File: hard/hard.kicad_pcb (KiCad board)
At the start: 2 copper layers, 315.6 x 117.5 mm, 177 parts, among them J1 USB_C_Receptacle_USB2.0, J2 RJ45_Shielded, J3 RJ45_Shielded, SW1 BOOT0, SW2 BOOT1, SW3 BOOT0, SW4 BOOT1, U1 STM32F401RETx, U2 USBLC6-2SC6, U3 AMS1117-3.3, U4 STM32F401RETx, Y1 XTAL_8M, Y3 XTAL_8M

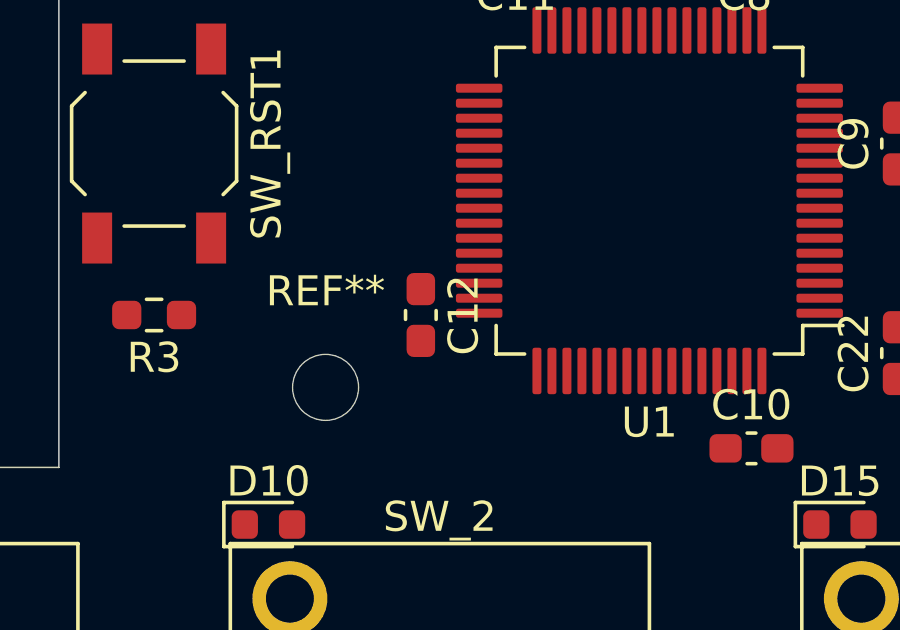
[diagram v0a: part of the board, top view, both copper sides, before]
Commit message: misc circuits
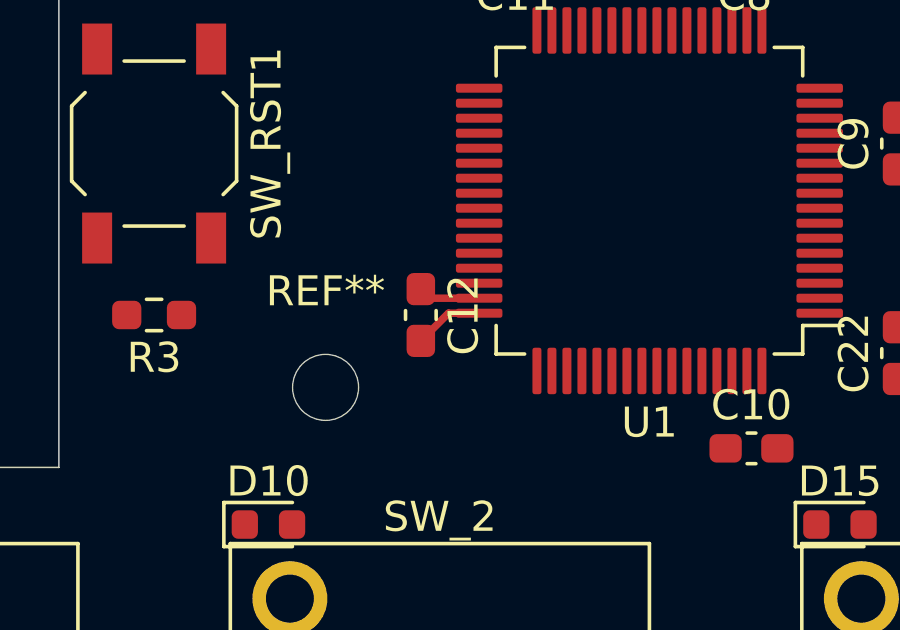
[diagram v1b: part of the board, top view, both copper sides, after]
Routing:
- net +3V3: track 0.00 -> 2.33 mm
- net GND: track 0.00 -> 2.07 mm

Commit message: gen2
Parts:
- removed C15, C17, C19, C20, C21, C22, C23: 0.1uF, Capacitor_SMD:C_0603_1608Metric_Pad1.08x0.95mm_HandSolder
- removed C16: 10uF, Capacitor_SMD:C_0603_1608Metric_Pad1.08x0.95mm_HandSolder
- removed C18: 4.7uF, Capacitor_SMD:C_0603_1608Metric_Pad1.08x0.95mm_HandSolder
- removed C24, C25: 12pF, Capacitor_SMD:C_0603_1608Metric_Pad1.08x0.95mm_HandSolder
- removed D10, D11, D12, D13, D14, D15, D16, D17, D18, D19, D20, D21, D22, D23, D24, D25, D26, D27, D29, D30, D31, D32, D33, D34, D35, D36, D37, D38, D39, D4, D40, D41, D42, D43, D44, D45, D46, D47, D48, D49, D5, D50, D51, D52, D53, D54, D55, D56, D57, D58, D59, D6, D60, D61, D62, D7, D8, D9: D, Diode_SMD:D_0603_1608Metric
- removed J3: RJ45_Shielded, Connector_RJ:RJ45_Ninigi_GE
- removed REF** (x8): MountingHole_2.2mm_M2, MountingHole:MountingHole_2.2mm_M2
- removed SW_0: SW_0, hard:Kailh_Choc_V2_1.00u_PCB
- removed SW_1: SW_1, hard:Kailh_Choc_V2_1.00u_PCB
- removed SW_10: SW_6, hard:Kailh_Choc_V2_1.00u_PCB
- removed SW_2: SW_2, hard:Kailh_Choc_V2_1.00u_PCB
- removed SW_3: SW_3, hard:Kailh_Choc_V2_1.00u_PCB
- removed SW_4: SW_4, hard:Kailh_Choc_V2_1.00u_PCB
- removed SW_5: SW_5, hard:Kailh_Choc_V2_1.00u_PCB
- removed SW_7: SW_7, hard:Kailh_Choc_V2_1.00u_PCB
- removed SW_8: SW_8, hard:Kailh_Choc_V2_1.00u_PCB
- removed SW_9: SW_9, hard:Kailh_Choc_V2_1.00u_PCB
- removed SW_A1: SW_A, hard:Kailh_Choc_V2_1.00u_PCB
- removed SW_B1: SW_B, hard:Kailh_Choc_V2_1.00u_PCB
- removed SW_BQ1: SW_BQ, hard:Kailh_Choc_V2_1.00u_PCB
- removed SW_BS1: SW_BS, hard:Kailh_Choc_V2_1.50u_PCB
- removed SW_C1: SW_C, hard:Kailh_Choc_V2_1.00u_PCB
- removed SW_CMM1: SW_CMM, hard:Kailh_Choc_V2_1.00u_PCB
- removed SW_CTRL1: SW_CTRL, hard:Kailh_Choc_V2_1.75u_PCB
- removed SW_D1: SW_D, hard:Kailh_Choc_V2_1.00u_PCB
- removed SW_DEL1: SW_DEL, hard:Kailh_Choc_V2_2.00u_PCB
- removed SW_E1: SW_E, hard:Kailh_Choc_V2_1.00u_PCB
- removed SW_ESC1: SW_ESC, hard:Kailh_Choc_V2_1.00u_PCB
- removed SW_F1: SW_F, hard:Kailh_Choc_V2_1.00u_PCB
- removed SW_FN1: SW_FN, hard:Kailh_Choc_V2_1.00u_PCB
- removed SW_G1: SW_G, hard:Kailh_Choc_V2_1.00u_PCB
- removed SW_H1: SW_H, hard:Kailh_Choc_V2_1.00u_PCB
- removed SW_HYPH1: SW_HYPH, hard:Kailh_Choc_V2_1.00u_PCB
- removed SW_I1: SW_I, hard:Kailh_Choc_V2_1.00u_PCB
- removed SW_J1: SW_J, hard:Kailh_Choc_V2_1.00u_PCB
- removed SW_K1: SW_K, hard:Kailh_Choc_V2_1.00u_PCB
- removed SW_L1: SW_L, hard:Kailh_Choc_V2_1.00u_PCB
- removed SW_LALT1: SW_LALT, hard:Kailh_Choc_V2_1.25u_PCB
- removed SW_LB1: SW_LB, hard:Kailh_Choc_V2_1.00u_PCB
- removed SW_LCMD1: SW_LCMD, hard:Kailh_Choc_V2_1.25u_PCB
- removed SW_LSFT1: SW_LSFT, hard:Kailh_Choc_V2_2.25u_PCB
- removed SW_LSPC1: SW_LSPC, hard:Kailh_Choc_V2_2.00u_PCB
- removed SW_M1: SW_M, hard:Kailh_Choc_V2_1.00u_PCB
- removed SW_N1: SW_N, hard:Kailh_Choc_V2_1.00u_PCB
- removed SW_O1: SW_O, hard:Kailh_Choc_V2_1.00u_PCB
- removed SW_P1: SW_P, hard:Kailh_Choc_V2_1.00u_PCB
- removed SW_PLUS1: SW_PLUS, hard:Kailh_Choc_V2_1.00u_PCB
- removed SW_PRD1: SW_PRD, hard:Kailh_Choc_V2_1.00u_PCB
- removed SW_Q1: SW_Q, hard:Kailh_Choc_V2_1.00u_PCB
- removed SW_R1: SW_R, hard:Kailh_Choc_V2_1.00u_PCB
- removed SW_RALT1: SW_RALT, hard:Kailh_Choc_V2_1.25u_PCB
- removed SW_RB1: SW_RB, hard:Kailh_Choc_V2_1.00u_PCB
- removed SW_RCMD1: SW_RCMD, hard:Kailh_Choc_V2_1.25u_PCB
- removed SW_RET1: SW_RET, hard:Kailh_Choc_V2_2.75u_PCB
- removed SW_RSFT1: SW_RSFT, hard:Kailh_Choc_V2_2.25u_PCB
- removed SW_RSPC1: SW_RSPC, hard:Kailh_Choc_V2_2.00u_PCB
- removed SW_RST1, SW_RST2: RST, Button_Switch_SMD:SW_SPST_TL3342
- removed SW_S1: SW_S, hard:Kailh_Choc_V2_1.00u_PCB
- removed SW_SEMI1: SW_SEMI, hard:Kailh_Choc_V2_1.00u_PCB
- removed SW_SLA1: SW_SLA, hard:Kailh_Choc_V2_1.00u_PCB
- removed SW_SQ1: SW_SQ, hard:Kailh_Choc_V2_1.00u_PCB
- removed SW_T1: SW_T, hard:Kailh_Choc_V2_1.00u_PCB
- removed SW_TAB1: SW_TAB, hard:Kailh_Choc_V2_1.50u_PCB
- removed SW_U1: SW_U, hard:Kailh_Choc_V2_1.00u_PCB
- removed SW_V1: SW_V, hard:Kailh_Choc_V2_1.00u_PCB
- removed SW_W1: SW_W, hard:Kailh_Choc_V2_1.00u_PCB
- removed SW_X1: SW_X, hard:Kailh_Choc_V2_1.00u_PCB
- removed SW_Y1: SW_Y, hard:Kailh_Choc_V2_1.00u_PCB
- removed SW_Z1: SW_Z, hard:Kailh_Choc_V2_1.00u_PCB
- removed Y3: XTAL_8M, Crystal:Crystal_SMD_3225-4Pin_3.2x2.5mm_HandSoldering
- added C3: 0.1uF, Capacitor_SMD:C_0402_1005Metric_Pad0.74x0.62mm_HandSolder, F.Cu at (175.8, 64.0)
- added C4: 0.1uF, Capacitor_SMD:C_0402_1005Metric_Pad0.74x0.62mm_HandSolder, F.Cu at (181.6, 63.0)
- added R10: 330Ohm, Resistor_SMD:R_0402_1005Metric_Pad0.72x0.64mm_HandSolder, F.Cu at (168.3, 45.7)
- added R9: 330Ohm, Resistor_SMD:R_0402_1005Metric_Pad0.72x0.64mm_HandSolder, F.Cu at (165.1, 46.4)
- added REF_M1: MountingHole_2.2mm_M2_DIN965, MountingHole:MountingHole_2.2mm_M2_DIN965, F.Cu at (188.0, 48.3)
- added REF_M2: MountingHole_2.2mm_M2_DIN965, MountingHole:MountingHole_2.2mm_M2_DIN965, F.Cu at (188.0, 62.9)
- added REF_M3: MountingHole_2.2mm_M2_DIN965, MountingHole:MountingHole_2.2mm_M2_DIN965, F.Cu at (153.0, 48.3)
- added REF_M4: MountingHole_2.2mm_M2_DIN965, MountingHole:MountingHole_2.2mm_M2_DIN965, F.Cu at (153.0, 62.9)
- added SW10: KEY_Q, hard:Kailh_Choc_V2_1.00u_PCB, F.Cu at (120.0, 89.5)
- added SW11: KEY_A, hard:Kailh_Choc_V2_1.00u_PCB, F.Cu at (125.3, 108.6)
- added SW12: KEY_OPTION, hard:Kailh_Choc_V2_1.25u_PCB, F.Cu at (136.7, 146.7)
- added SW13: KEY_2, hard:Kailh_Choc_V2_1.00u_PCB, F.Cu at (129.5, 70.5)
- added SW14: KEY_Z, hard:Kailh_Choc_V2_1.00u_PCB, F.Cu at (134.3, 127.6)
- added SW15: KEY_W, hard:Kailh_Choc_V2_1.00u_PCB, F.Cu at (139.1, 89.5)
- added SW16: KEY_S, hard:Kailh_Choc_V2_1.00u_PCB, F.Cu at (144.3, 108.6)
- added SW17: KEY_COMMAND, hard:Kailh_Choc_V2_1.25u_PCB, F.Cu at (160.5, 146.7)
- added SW18: KEY_3, hard:Kailh_Choc_V2_1.00u_PCB, F.Cu at (148.6, 70.5)
- added SW19: KEY_X, hard:Kailh_Choc_V2_1.00u_PCB, F.Cu at (153.4, 127.6)
- added SW20: KEY_E, hard:Kailh_Choc_V2_1.00u_PCB, F.Cu at (158.1, 89.5)
- added SW21: KEY_D, hard:Kailh_Choc_V2_1.00u_PCB, F.Cu at (163.4, 108.6)
- added SW22: KEY_4, hard:Kailh_Choc_V2_1.00u_PCB, F.Cu at (167.6, 70.5)
- added SW23: KEY_C, hard:Kailh_Choc_V2_1.00u_PCB, F.Cu at (172.4, 127.6)
- added SW24: KEY_R, hard:Kailh_Choc_V2_1.00u_PCB, F.Cu at (177.2, 89.5)
- added SW25: KEY_F, hard:Kailh_Choc_V2_1.00u_PCB, F.Cu at (182.4, 108.6)
- added SW26: KEY_5, hard:Kailh_Choc_V2_1.00u_PCB, F.Cu at (186.7, 70.5)
- added SW27: KEY_SPACE, hard:Kailh_Choc_V2_2.00u_PCB, F.Cu at (195.6, 146.7)
- added SW28: KEY_V, hard:Kailh_Choc_V2_1.00u_PCB, F.Cu at (191.5, 127.6)
- added SW29: KEY_T, hard:Kailh_Choc_V2_1.00u_PCB, F.Cu at (196.2, 89.5)
- added SW30: KEY_G, hard:Kailh_Choc_V2_1.00u_PCB, F.Cu at (201.5, 108.6)
- added SW31: KEY_6, hard:Kailh_Choc_V2_1.00u_PCB, F.Cu at (205.7, 70.5)
- added SW32: KEY_B, hard:Kailh_Choc_V2_1.00u_PCB, F.Cu at (210.5, 127.6)
- added SW5: KEY_LFN, hard:Kailh_Choc_V2_1.00u_PCB, F.Cu at (91.5, 146.7)
- added SW6: KEY_TAB, hard:Kailh_Choc_V2_1.50u_PCB, F.Cu at (96.2, 89.5)
- added SW7: KEY_ESCAPE, hard:Kailh_Choc_V2_1.00u_PCB, F.Cu at (91.4, 70.5)
- added SW8: KEY_CONTROL, hard:Kailh_Choc_V2_1.25u_PCB, F.Cu at (112.9, 146.7)
- added SW9: KEY_1, hard:Kailh_Choc_V2_1.00u_PCB, F.Cu at (110.5, 70.5)
- added U5: STM32L412RBTx, Package_QFP:LQFP-64_10x10mm_P0.5mm, F.Cu at (164.7, 55.4)
- C1: value 12pF -> 0.1uF; footprint Capacitor_SMD:C_0603_1608Metric_Pad1.08x0.95mm_HandSolder -> Capacitor_SMD:C_0402_1005Metric_Pad0.74x0.62mm_HandSolder
- C10, C11, C12, C14, C8, C9: footprint Capacitor_SMD:C_0603_1608Metric_Pad1.08x0.95mm_HandSolder -> Capacitor_SMD:C_0402_1005Metric_Pad0.74x0.62mm_HandSolder
- C13: value 10uF -> 0.1uF; footprint Capacitor_SMD:C_0603_1608Metric_Pad1.08x0.95mm_HandSolder -> Capacitor_SMD:C_0402_1005Metric_Pad0.74x0.62mm_HandSolder
- C2: value 12pF -> 1uF
- C5: value 0.1uF -> 1uF
- C6: value 4.7uF -> 10pF; footprint Capacitor_SMD:C_0603_1608Metric_Pad1.08x0.95mm_HandSolder -> Capacitor_SMD:C_0402_1005Metric_Pad0.74x0.62mm_HandSolder
- C7: value 0.1uF -> 10pF; footprint Capacitor_SMD:C_0603_1608Metric_Pad1.08x0.95mm_HandSolder -> Capacitor_SMD:C_0402_1005Metric_Pad0.74x0.62mm_HandSolder
- D1: footprint Diode_SMD:D_0603_1608Metric -> Diode_SMD:D_SOD-123
- D2: value D -> STATUS1; footprint Diode_SMD:D_0603_1608Metric -> LED_SMD:LED_0603_1608Metric_Pad1.05x0.95mm_HandSolder
- D3: value D -> STATUS2; footprint Diode_SMD:D_0603_1608Metric -> LED_SMD:LED_0603_1608Metric_Pad1.05x0.95mm_HandSolder
- F1: footprint Fuse:Fuse_0603_1608Metric_Pad1.05x0.95mm_HandSolder -> Fuse:Fuse_0805_2012Metric_Pad1.15x1.40mm_HandSolder
- J2: value RJ45_Shielded -> RJ45_LED_Shielded; footprint Connector_RJ:RJ45_Ninigi_GE -> Connector_RJ:RJ45_Hanrun_HR911105A
- R1, R2: value 10kohm -> 5.1kOhm; footprint Resistor_SMD:R_0603_1608Metric_Pad0.98x0.95mm_HandSolder -> Resistor_SMD:R_0402_1005Metric_Pad0.72x0.64mm_HandSolder
- R3: value 4.7kohm -> R; footprint Resistor_SMD:R_0603_1608Metric_Pad0.98x0.95mm_HandSolder -> Resistor_SMD:R_0402_1005Metric_Pad0.72x0.64mm_HandSolder
- R4: value 5.1kohm -> R; footprint Resistor_SMD:R_0603_1608Metric_Pad0.98x0.95mm_HandSolder -> Resistor_SMD:R_0402_1005Metric_Pad0.72x0.64mm_HandSolder
- R5: value 5.1kohm -> 4.7kOhm; footprint Resistor_SMD:R_0603_1608Metric_Pad0.98x0.95mm_HandSolder -> Resistor_SMD:R_0402_1005Metric_Pad0.72x0.64mm_HandSolder
- R6: value 4.7kohm -> 4.7kOhm; footprint Resistor_SMD:R_0603_1608Metric_Pad0.98x0.95mm_HandSolder -> Resistor_SMD:R_0402_1005Metric_Pad0.72x0.64mm_HandSolder
- R7: value 10kohm -> 2.2kOhm; footprint Resistor_SMD:R_0603_1608Metric_Pad0.98x0.95mm_HandSolder -> Resistor_SMD:R_0402_1005Metric_Pad0.72x0.64mm_HandSolder
- R8: value 10kohm -> 3.3kOhm; footprint Resistor_SMD:R_0603_1608Metric_Pad0.98x0.95mm_HandSolder -> Resistor_SMD:R_0402_1005Metric_Pad0.72x0.64mm_HandSolder
- SW1: value BOOT0 -> SW_RST; footprint Button_Switch_SMD:SW_SPDT_PCM12 -> Button_Switch_SMD:SW_SPST_CK_KXT3
- SW2: value BOOT1 -> SW_BOOT0; footprint Button_Switch_SMD:SW_SPDT_PCM12 -> Button_Switch_SMD:SW_SPST_CK_KXT3
- SW3: value BOOT0 -> KEY_CAPSLOCK; footprint Button_Switch_SMD:SW_SPDT_PCM12 -> hard:Kailh_Choc_V2_1.75u_PCB
- SW4: value BOOT1 -> KEY_LSHIFT; footprint Button_Switch_SMD:SW_SPDT_PCM12 -> hard:Kailh_Choc_V2_2.25u_PCB
- U1: value STM32F401RETx -> THVD1451D; footprint Package_QFP:LQFP-64_10x10mm_P0.5mm -> Package_SO:SOIC-8_3.9x4.9mm_P1.27mm
- U3: value AMS1117-3.3 -> MIC5504-3.3YM5; footprint Package_TO_SOT_SMD:SOT-223-3_TabPin2 -> Package_TO_SOT_SMD:SOT-23-5
- U4: value STM32F401RETx -> STLinkV3; footprint Package_QFP:LQFP-64_10x10mm_P0.5mm -> hard:IDC-Header_2x07_P1.27mm_Vertical
- Y1: value XTAL_8M -> 8MHz
- moved SW4 937.1 mm to (103.4, 127.6), turned to 0 degrees
- moved SW3 927.6 mm to (98.6, 108.6), turned to 0 degrees
- moved R6 894.3 mm to (158.1, 48.3)
- moved U4 886.1 mm to (148.6, 62.1)
- moved C5 854.3 mm to (183.1, 63.0), turned to 270 degrees
- moved R8 842.4 mm to (186.1, 60.3)
- moved R7 834.9 mm to (183.5, 60.3)
- moved R5 749.9 mm to (158.1, 47.0)
- moved SW2 748.8 mm to (148.0, 50.2), turned to 0 degrees
- moved SW1 738.7 mm to (148.0, 47.6), turned to 0 degrees
- moved C7 737.6 mm to (153.5, 59.7), turned to 180 degrees
- moved C13 733.6 mm to (157.9, 51.3), turned to 225 degrees
- moved J2 732.5 mm to (195.6, 59.4), turned to 90 degrees
- moved Y1 731.8 mm to (153.5, 56.3)
- moved J1 729.0 mm to (178.3, 49.3)
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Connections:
- net +5V renamed Net-(F1-Pad2)
- C1 pad 1: /L_XTAL_8M_B -> +3V3
- C13 pad 1: Net-(C13-Pad1) -> GND
- C13 pad 2: GND -> +3V3
- C14 pad 1: Net-(C13-Pad1) -> /V_SHARED
- C2 pad 1: /L_XTAL_8M_A -> Net-(C2-Pad1)
- C6 pad 1: Net-(C6-Pad1) -> /XTAL_A
- C7 pad 1: GND -> /XTAL_B
- C7 pad 2: +3V3 -> GND
- D1 pad 1: /COL1L -> Net-(C2-Pad1)
- D1 pad 2: Net-(D1-Pad2) -> /V_SHARED
- D2 pad 1: /COL1L -> Net-(D2-Pad1)
- D3 pad 1: /COL1L -> Net-(D3-Pad1)
- F1 pad 1: Net-(C13-Pad1) -> /V_SHARED
- J2 pad 1: (no net) -> /ETH_TX-
- J2 pad 2: (no net) -> /ETH_TX+
- J2 pad 3: (no net) -> /ETH_RX-
- J2 pad 4: (no net) -> /V_SHARED
- J2 pad 5: (no net) -> /V_SHARED
- J2 pad 6: (no net) -> /ETH_RX+
- J2 pad 7: (no net) -> GND
- J2 pad 8: (no net) -> GND
- R1 pad 1: /R_BOOT0 -> Net-(J1-PadB5)
- R2 pad 1: /R_BOOT1 -> Net-(J1-PadA5)
- R3 pad 1: +3V3 -> GND
- R3 pad 2: Net-(R3-Pad2) -> Net-(J2-Pad9)
- R4 pad 1: Net-(J1-PadB5) -> GND
- R4 pad 2: GND -> Net-(J2-Pad11)
- R5 pad 1: Net-(J1-PadA5) -> +3V3
- R5 pad 2: GND -> /NRST
- R6 pad 1: +3V3 -> Net-(R6-Pad1)
- R6 pad 2: Net-(R6-Pad2) -> GND
- R7 pad 1: /L_BOOT0 -> Net-(C2-Pad1)
- R7 pad 2: GND -> /VBUS_DETECT
- R8 pad 1: /L_BOOT1 -> /VBUS_DETECT
- SW1 pad 2: /R_BOOT0 -> /NRST
- SW2 pad 1: GND -> +3V3
- SW2 pad 2: /R_BOOT1 -> Net-(R6-Pad1)
- SW3 pad 2: /L_BOOT0 -> /KEY_CAPSLOCK
- SW4 pad 2: /L_BOOT1 -> /KEY_LSHIFT
- U1 pad 2: (no net) -> /RX
- U1 pad 3: (no net) -> /TX
- U1 pad 4: (no net) -> GND
- U1 pad 5: /L_XTAL_8M_A -> /ETH_TX-
- U1 pad 6: /L_XTAL_8M_B -> /ETH_TX+
- U1 pad 7: Net-(R3-Pad2) -> /ETH_RX-
- U1 pad 8: (no net) -> /ETH_RX+
- U2 pad 1: (no net) -> /D+
- U2 pad 3: (no net) -> /D-
- U2 pad 5: +3V3 -> /V_SHARED
- U3 pad 1: GND -> Net-(C2-Pad1)
- U3 pad 2: +3V3 -> GND
- U3 pad 3: Net-(C13-Pad1) -> Net-(C2-Pad1)
- U4 pad 1: +3V3 -> (no net)
- U4 pad 10: (no net) -> /JTDI
- U4 pad 11: (no net) -> GND
- U4 pad 12: GND -> /NRST
- U4 pad 13: +3V3 -> /VPC_TX
- U4 pad 14: (no net) -> /VPC_RX
- U4 pad 3: (no net) -> +3V3
- U4 pad 4: (no net) -> /JTMS
- U4 pad 5: /R_XTAL_8M_A -> GND
- U4 pad 6: /R_XTAL_8M_B -> /JTCK
- U4 pad 7: Net-(R6-Pad2) -> GND
- U4 pad 8: (no net) -> /JTDO
- U4 pad 9: (no net) -> /JTCK
- Y1 pad 1: /L_XTAL_8M_B -> /XTAL_A
- Y1 pad 3: /L_XTAL_8M_A -> /XTAL_B
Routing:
- net GND: track 2.07 -> 214.1 mm, vias 0 -> 12
- net /KEY_LFN: track 0.00 -> 129.3 mm, vias 0 -> 1
- net /KEY_B: track 0.00 -> 123.1 mm, vias 0 -> 1
- net /KEY_CONTROL: track 0.00 -> 119.2 mm, vias 0 -> 1
- net /KEY_SPACE: track 0.00 -> 114.3 mm, vias 0 -> 1
- net /KEY_OPTION: track 0.00 -> 114.3 mm, vias 0 -> 1
- net +3V3: track 2.33 -> 115.7 mm, vias 0 -> 10
- net /KEY_V: track 0.00 -> 109.1 mm, vias 0 -> 1
- net /KEY_CAPSLOCK: track 0.00 -> 102.6 mm
- net /KEY_Q: track 0.00 -> 101.6 mm, vias 0 -> 2
- net /KEY_COMMAND: track 0.00 -> 100.8 mm, vias 0 -> 1
- net /KEY_G: track 0.00 -> 97.6 mm, vias 0 -> 1
- net /KEY_A: track 0.00 -> 94.6 mm, vias 0 -> 4
- net /KEY_X: track 0.00 -> 90.9 mm, vias 0 -> 2
- net /KEY_C: track 0.00 -> 90.9 mm, vias 0 -> 3
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- added copper zone on B.Cu, net GND
- added copper zone on F.Cu, net GND
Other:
- board size 315.6 x 117.5 mm -> 138.1 x 118.7 mm
- net class Default: trace_width 0.25 -> 0.2; via_dia 0.8 -> 0.5; via_drill 0.4 -> 0.3
